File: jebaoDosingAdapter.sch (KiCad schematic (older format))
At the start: 4 parts, among them J1 Conn_01x05_Male, J2 Conn_01x02_Male, J3 6P6C, U1 ULN2803A

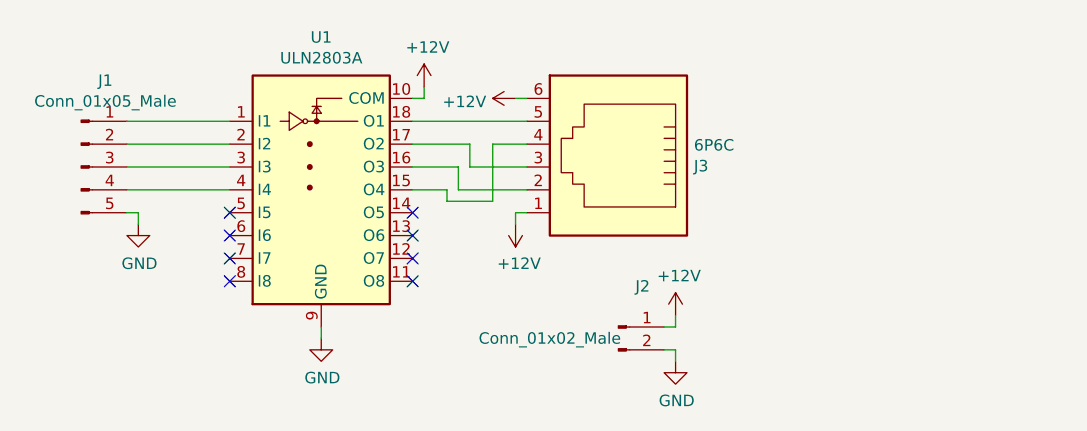
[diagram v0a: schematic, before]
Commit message: Add images and updated gerbers
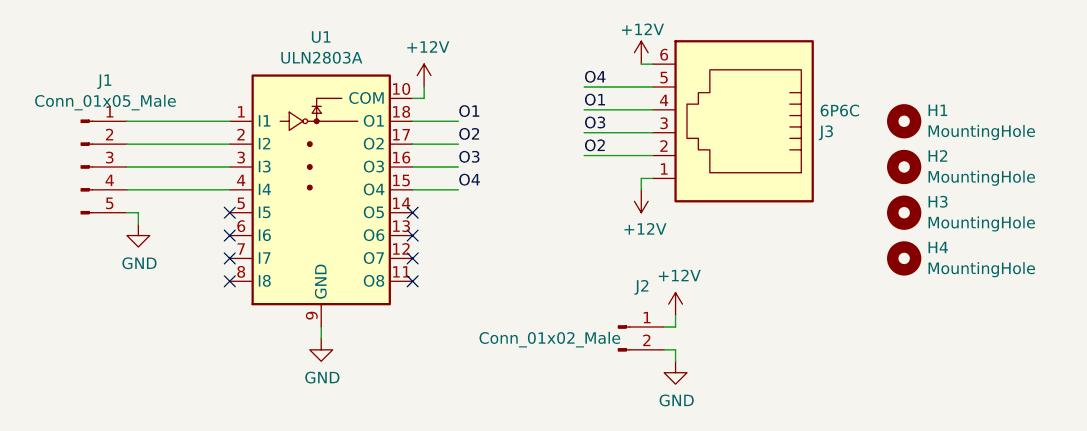
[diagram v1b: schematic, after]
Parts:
- added H1, H2, H3, H4: MountingHole, MountingHole:MountingHole_3.2mm_M3, symbol Mechanical:MountingHole
- J1: footprint Connector_PinHeader_2.54mm:PinHeader_1x05_P2.54mm_Vertical -> Connector_JST:JST_XH_B05B-XH-A_1x05_P2.50mm_Vertical
- J2: footprint Connector_PinHeader_2.54mm:PinHeader_1x02_P2.54mm_Vertical -> Connector_JST:JST_XH_B02B-XH-A_1x02_P2.50mm_Vertical
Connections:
- net O1: now reaches J3.4
- net O1: now also U1.18 (O1); no longer U1.15 (O4)
- net O2: now reaches J3.2
- net O2: now also U1.17 (O2); no longer U1.16 (O3)
- net O3: now reaches J3.3
- net O3: now also U1.16 (O3); no longer U1.17 (O2)
- net O4: now reaches J3.5
- net O4: now also U1.15 (O4); no longer U1.18 (O1)
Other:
- moved on the sheet: J3
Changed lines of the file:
@@
 EESchema Schematic File Version 4
 LIBS:jebaoDosingAdapter-cache
-EELAYER 29 0
+EELAYER 26 0
 EELAYER END
 $Descr A4 11693 8268
@@
 $EndComp
 $Comp
-L Connector:6P6C J3
-U 1 1 5D71C0A6
-P 6600 2750
-F 0 "J3" H 6270 2754 50  0000 R CNN
-F 1 "6P6C" H 6270 2845 50  0000 R CNN
-F 2 "jebaoDosingAdapter:RJ11" V 6600 2775 50  0001 C CNN
-F 3 "~" V 6600 2775 50  0001 C CNN
-	1    6600 2750
-	-1   0    0    -1
-$EndComp
-$Comp
 L Connector:Conn_01x02_Male J2
 U 1 1 5D71C249
@@
 F 0 "J2" H 6706 3628 50  0000 C CNN
 F 1 "Conn_01x02_Male" H 6300 3400 50  0000 C CNN
-F 2 "Connector_PinHeader_2.54mm:PinHeader_1x02_P2.54mm_Vertical" H 6600 3450 50  0001 C CNN
+F 2 "Connector_JST:JST_XH_B02B-XH-A_1x02_P2.50mm_Vertical" H 6600 3450 50  0001 C CNN
 F 3 "~" H 6600 3450 50  0001 C CNN
 	1    6600 3450
@@
 F 0 "J1" H 4356 3128 50  0000 C CNN
 F 1 "Conn_01x05_Male" H 4356 3037 50  0000 C CNN
-F 2 "Connector_PinHeader_2.54mm:PinHeader_1x05_P2.54mm_Vertical" H 4250 2750 50  0001 C CNN
+F 2 "Connector_JST:JST_XH_B05B-XH-A_1x05_P2.50mm_Vertical" H 4250 2750 50  0001 C CNN
 F 3 "~" H 4250 2750 50  0001 C CNN
 	1    4250 2750
@@
 L power:+12V #PWR04
 U 1 1 5D71CEE9
-P 6150 3000
-F 0 "#PWR04" H 6150 2850 50  0001 C CNN
-F 1 "+12V" H 6165 3173 50  0000 C CNN
-F 2 "" H 6150 3000 50  0001 C CNN
-F 3 "" H 6150 3000 50  0001 C CNN
-	1    6150 3000
+P 6700 2850
+F 0 "#PWR04" H 6700 2700 50  0001 C CNN
+F 1 "+12V" H 6715 3023 50  0000 C CNN
+F 2 "" H 6700 2850 50  0001 C CNN
+F 3 "" H 6700 2850 50  0001 C CNN
+	1    6700 2850
 	1    0    0    1
 $EndComp
 Wire Wire Line
-	6150 3000 6150 2950
-Wire Wire Line
-	6150 2950 6200 2950
+	6700 2850 6700 2800
+Wire Wire Line
+	6700 2800 6750 2800
 $Comp
 L power:+12V #PWR05
 U 1 1 5D7302C7
-P 6150 2450
-F 0 "#PWR05" H 6150 2300 50  0001 C CNN
-F 1 "+12V" V 6165 2578 50  0000 L CNN
-F 2 "" H 6150 2450 50  0001 C CNN
-F 3 "" H 6150 2450 50  0001 C CNN
-	1    6150 2450
-	0    -1   1    0
-$EndComp
-Wire Wire Line
-	6200 2450 6150 2450
-Wire Wire Line
-	6200 2550 5700 2550
-Wire Wire Line
-	6200 2750 5950 2750
-Wire Wire Line
-	5950 2750 5950 2650
-Wire Wire Line
-	5950 2650 5700 2650
-Wire Wire Line
-	6200 2850 5900 2850
-Wire Wire Line
-	5900 2850 5900 2750
-Wire Wire Line
-	5900 2750 5700 2750
-Wire Wire Line
-	6200 2650 6050 2650
-Wire Wire Line
-	6050 2650 6050 2900
-Wire Wire Line
-	6050 2900 5850 2900
-Wire Wire Line
-	5850 2900 5850 2850
-Wire Wire Line
-	5850 2850 5700 2850
+P 6700 2300
+F 0 "#PWR05" H 6700 2150 50  0001 C CNN
+F 1 "+12V" H 6600 2450 50  0000 L CNN
+F 2 "" H 6700 2300 50  0001 C CNN
+F 3 "" H 6700 2300 50  0001 C CNN
+	1    6700 2300
+	-1   0    0    -1
+$EndComp
+Wire Wire Line
+	6750 2300 6700 2300
+$Comp
+L Mechanical:MountingHole H1
+U 1 1 5D9A0E71
+P 7850 2550
+F 0 "H1" H 7950 2596 50  0000 L CNN
+F 1 "MountingHole" H 7950 2505 50  0000 L CNN
+F 2 "MountingHole:MountingHole_3.2mm_M3" H 7850 2550 50  0001 C CNN
+F 3 "~" H 7850 2550 50  0001 C CNN
+	1    7850 2550
+	1    0    0    -1
+$EndComp
+$Comp
+L Mechanical:MountingHole H2
+U 1 1 5D9A0EAC
+P 7850 2750
+F 0 "H2" H 7950 2796 50  0000 L CNN
+F 1 "MountingHole" H 7950 2705 50  0000 L CNN
+F 2 "MountingHole:MountingHole_3.2mm_M3" H 7850 2750 50  0001 C CNN
+F 3 "~" H 7850 2750 50  0001 C CNN
+	1    7850 2750
+	1    0    0    -1
+$EndComp
+$Comp
+L Mechanical:MountingHole H3
+U 1 1 5D9A0ED0
+P 7850 2950
+F 0 "H3" H 7950 2996 50  0000 L CNN
+F 1 "MountingHole" H 7950 2905 50  0000 L CNN
+F 2 "MountingHole:MountingHole_3.2mm_M3" H 7850 2950 50  0001 C CNN
+F 3 "~" H 7850 2950 50  0001 C CNN
+	1    7850 2950
+	1    0    0    -1
+$EndComp
+$Comp
+L Mechanical:MountingHole H4
+U 1 1 5D9A0EFA
+P 7850 3150
+F 0 "H4" H 7950 3196 50  0000 L CNN
+F 1 "MountingHole" H 7950 3105 50  0000 L CNN
+F 2 "MountingHole:MountingHole_3.2mm_M3" H 7850 3150 50  0001 C CNN
+F 3 "~" H 7850 3150 50  0001 C CNN
+	1    7850 3150
+	1    0    0    -1
+$EndComp
+$Comp
+L Connector:6P6C J3
+U 1 1 5D71C0A6
+P 7150 2600
+F 0 "J3" H 6820 2604 50  0000 R CNN
+F 1 "6P6C" H 6820 2695 50  0000 R CNN
+F 2 "jebaoDosingAdapter:RJ11" V 7150 2625 50  0001 C CNN
+F 3 "~" V 7150 2625 50  0001 C CNN
+	1    7150 2600
+	-1   0    0    -1
+$EndComp
+Wire Wire Line
+	5700 2550 5900 2550
+Wire Wire Line
+	5700 2650 5900 2650
+Wire Wire Line
+	5700 2750 5900 2750
+Wire Wire Line
+	5700 2850 5900 2850
+Wire Wire Line
+	6750 2400 6450 2400
+Wire Wire Line
+	6750 2500 6450 2500
+Wire Wire Line
+	6750 2600 6450 2600
+Wire Wire Line
+	6750 2700 6450 2700
+Text Label 5900 2550 0    50   ~ 0
+O1
+Text Label 6450 2500 0    50   ~ 0
+O1
+Text Label 5900 2650 0    50   ~ 0
+O2
+Text Label 6450 2700 0    50   ~ 0
+O2
+Text Label 5900 2750 0    50   ~ 0
+O3
+Text Label 6450 2600 0    50   ~ 0
+O3
+Text Label 5900 2850 0    50   ~ 0
+O4
+Text Label 6450 2400 0    50   ~ 0
+O4
 $EndSCHEMATC
